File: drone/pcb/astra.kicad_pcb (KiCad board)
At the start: 4 copper layers, 44.6 x 44.6 mm, 93 parts, among them J1 Conn_01x02_Pin, J2 Conn_02x11_Odd_Even, J3 Conn_01x04_MountingPin, J4 Conn_01x04_MountingPin, M1 Motor_DC, M2 Motor_DC, M3 Motor_DC, M4 Motor_DC, Q1 AO3400A, Q2 AO3400A, Q3 AO3400A, Q4 AO3400A, SW1 SW_Push, SW2 SW_Push, SW3 SW_Push, U1 TLV1117LV33DCYR, U2 W25Q64JVSSIQ_C179171, U3 STM32H750VBTx, U4 BMP388, U5 NRF24L01_Breakout, U7 BMI270, U8 HYCW110-TF10-180B, Y1 25 MHz

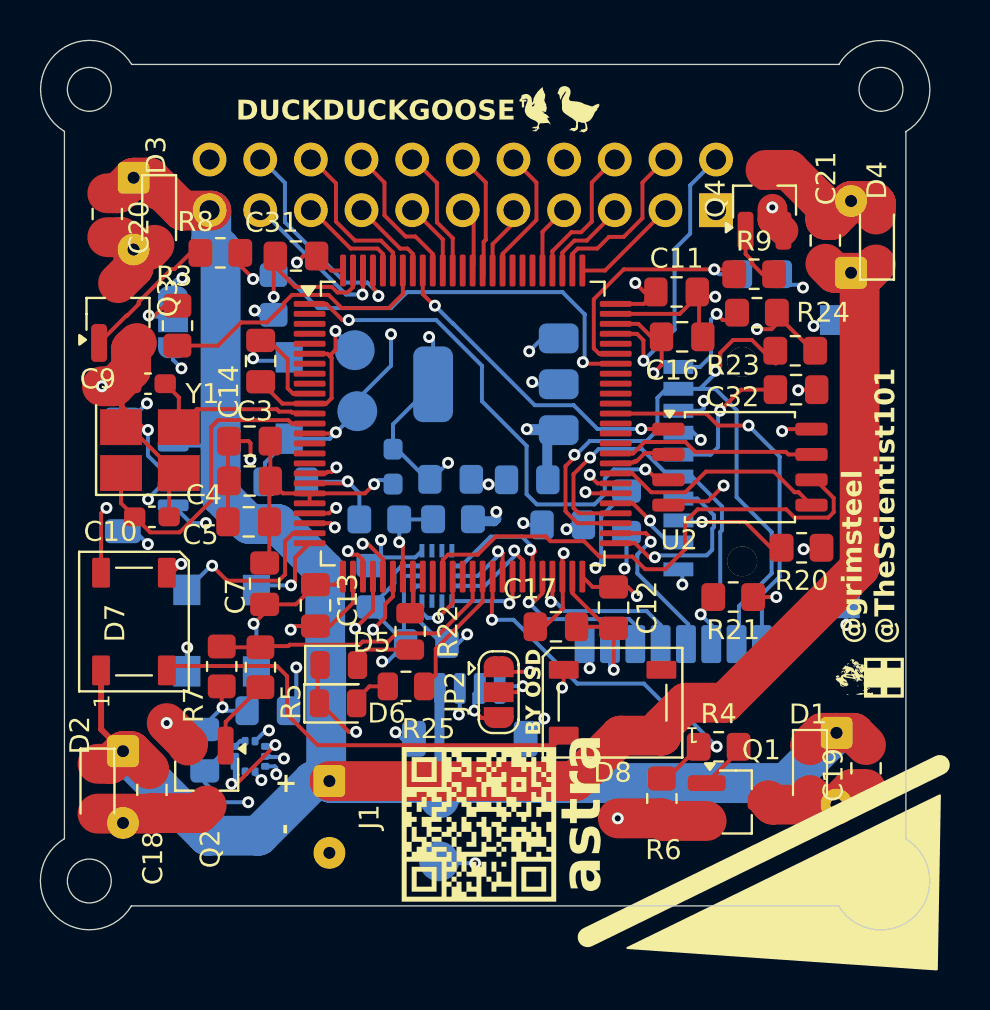
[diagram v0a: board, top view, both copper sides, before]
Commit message: [pcb] manufacturing constraints and cleanup
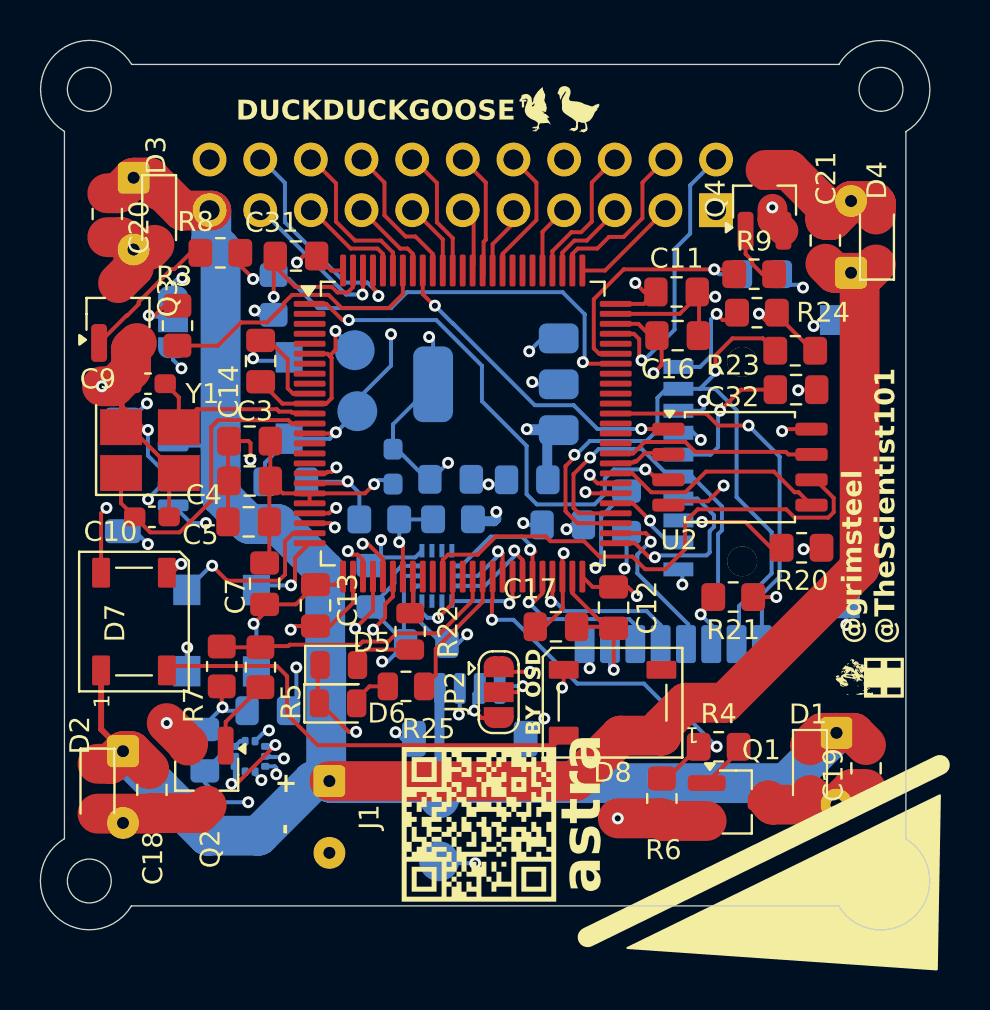
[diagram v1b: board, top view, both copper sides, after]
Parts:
- moved C16 0.24 mm to (155.4, 50.3)
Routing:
- net GND: track 132.0 -> 126.1 mm
- net +3.3V: track 73.6 -> 71.0 mm
- net DDG_MAGIC_7: track 3.46 -> 2.80 mm
- net BTN1: track 4.61 -> 4.00 mm
- net RST: track 26.0 -> 25.5 mm
- net UART4_RX: track 12.9 -> 12.3 mm
- net BAR_CS: track 16.0 -> 15.4 mm
- net SD_CD: track 4.06 -> 3.55 mm
- net Net-(C16-Pad2): track 19.7 -> 19.2 mm
